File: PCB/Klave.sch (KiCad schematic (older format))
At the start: 83 parts

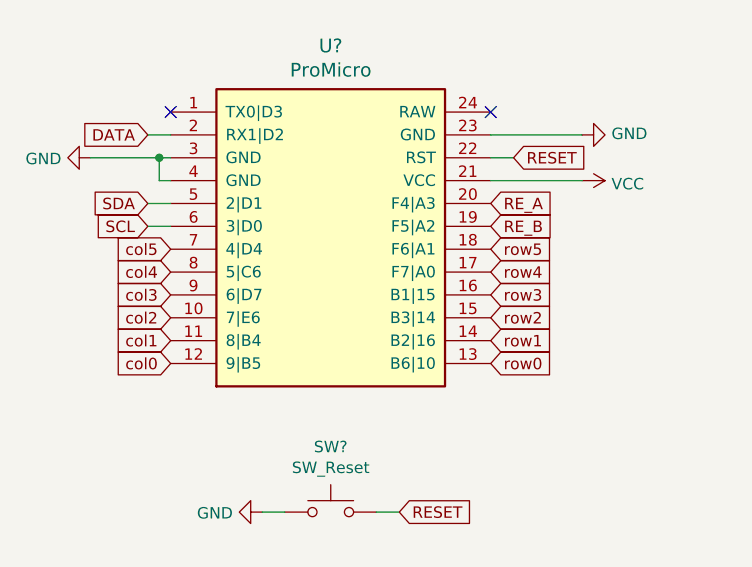
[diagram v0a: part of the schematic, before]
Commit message: Edit schematic
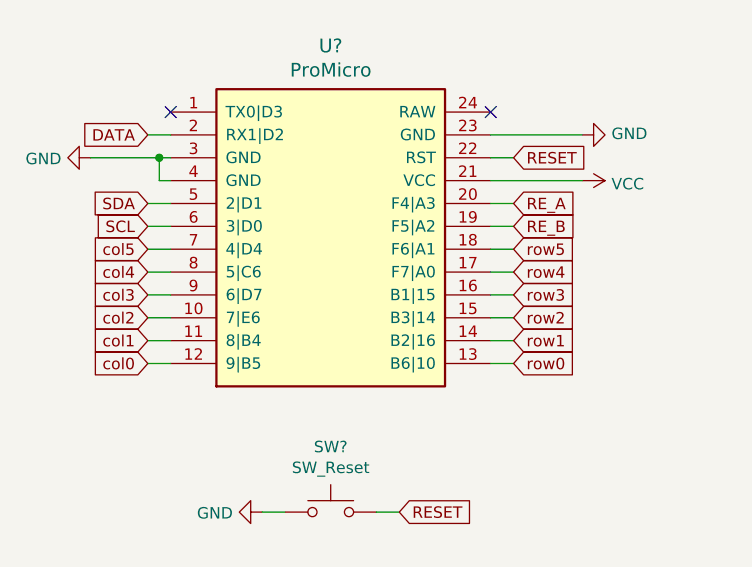
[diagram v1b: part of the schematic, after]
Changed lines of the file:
@@
 Text GLabel 6500 3600 0    50   Input ~ 0
 row3
-Text GLabel 1150 2550 0    50   Input ~ 0
+Text GLabel 1050 2550 0    50   Input ~ 0
 col0
-Text GLabel 1150 2450 0    50   Input ~ 0
+Text GLabel 1050 2450 0    50   Input ~ 0
 col1
-Text GLabel 1150 2350 0    50   Input ~ 0
+Text GLabel 1050 2350 0    50   Input ~ 0
 col2
-Text GLabel 1150 2250 0    50   Input ~ 0
+Text GLabel 1050 2250 0    50   Input ~ 0
 col3
-Text GLabel 2550 2550 2    50   Input ~ 0
+Text GLabel 2650 2550 2    50   Input ~ 0
 row0
-Text GLabel 2550 2450 2    50   Input ~ 0
+Text GLabel 2650 2450 2    50   Input ~ 0
 row1
-Text GLabel 2550 2350 2    50   Input ~ 0
+Text GLabel 2650 2350 2    50   Input ~ 0
 row2
-Text GLabel 2550 2250 2    50   Input ~ 0
+Text GLabel 2650 2250 2    50   Input ~ 0
 row3
-Text GLabel 2550 2150 2    50   Input ~ 0
+Text GLabel 2650 2150 2    50   Input ~ 0
 row4
-Text GLabel 1150 2150 0    50   Input ~ 0
+Text GLabel 1050 2150 0    50   Input ~ 0
 col4
-Text GLabel 1150 2050 0    50   Input ~ 0
+Text GLabel 1050 2050 0    50   Input ~ 0
 col5
 $Comp
@@
 Text GLabel 6500 4700 0    50   Input ~ 0
 row5
-Text GLabel 2550 2050 2    50   Input ~ 0
+Text GLabel 2650 2050 2    50   Input ~ 0
 row5
 $Comp
@@
 Wire Wire Line
 	9600 5750 9250 5750
-Text GLabel 2550 1850 2    50   Input ~ 0
+Text GLabel 2650 1850 2    50   Input ~ 0
 RE_A
-Text GLabel 2550 1950 2    50   Input ~ 0
+Text GLabel 2650 1950 2    50   Input ~ 0
 RE_B
 Text GLabel 9500 5850 0    50   Input ~ 0
@@
 Wire Wire Line
 	7050 4450 6950 4450
+Wire Wire Line
+	1050 2050 1150 2050
+Wire Wire Line
+	1150 2150 1050 2150
+Wire Wire Line
+	1050 2250 1150 2250
+Wire Wire Line
+	1050 2350 1150 2350
+Wire Wire Line
+	1150 2450 1050 2450
+Wire Wire Line
+	1050 2550 1150 2550
+Wire Wire Line
+	2550 2550 2650 2550
+Wire Wire Line
+	2650 2450 2550 2450
+Wire Wire Line
+	2550 2350 2650 2350
+Wire Wire Line
+	2650 2250 2550 2250
+Wire Wire Line
+	2550 2150 2650 2150
+Wire Wire Line
+	2650 2050 2550 2050
+Wire Wire Line
+	2550 1950 2650 1950
+Wire Wire Line
+	2650 1850 2550 1850
 $EndSCHEMATC
